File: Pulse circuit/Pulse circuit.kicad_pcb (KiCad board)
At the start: 4 copper layers, 8 parts, among them U1 module_max30102, U2 module_max30102, U3 DOIT-ESP32-DEVKIT-V1

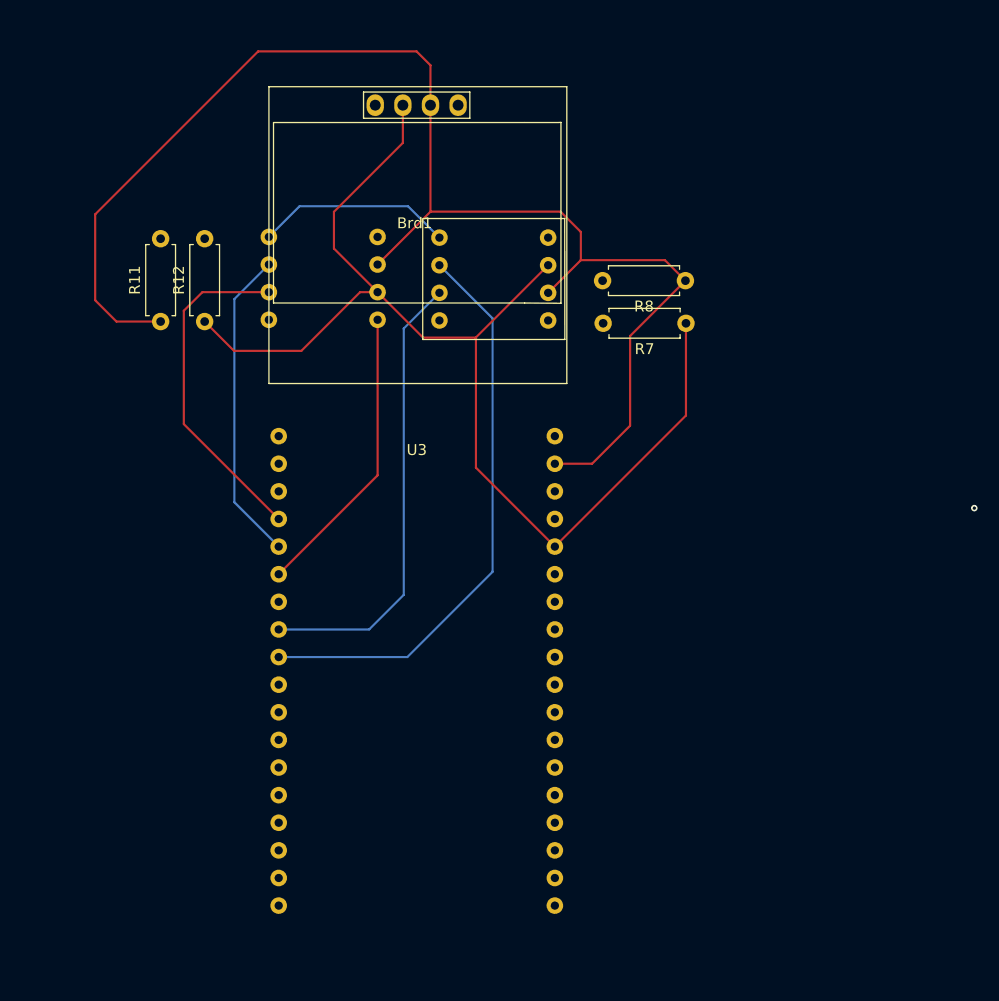
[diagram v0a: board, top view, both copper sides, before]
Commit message: Made some changes
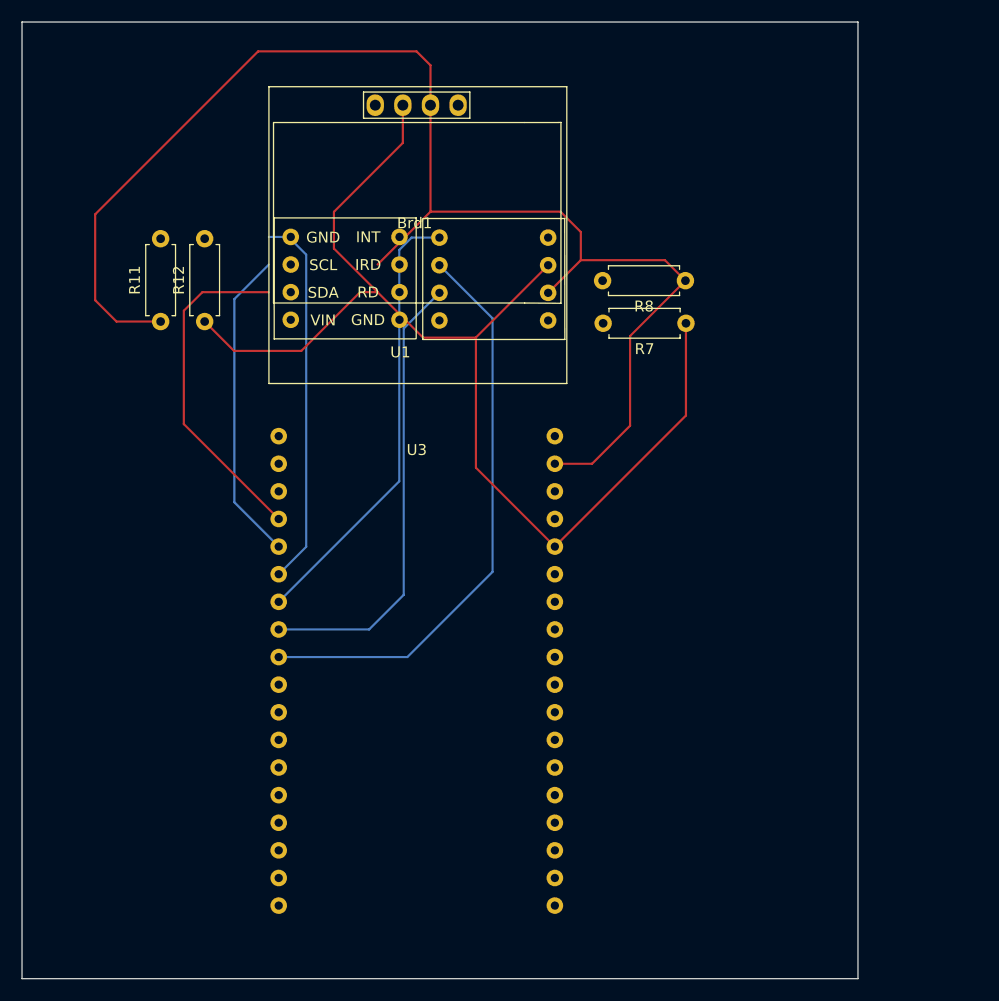
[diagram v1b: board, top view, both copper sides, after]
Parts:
- U1: moved to F.Cu
- moved U1 15.3 mm to (136.7, 74.7), turned to 0 degrees
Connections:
- U1 pad 8: INT5v -> INT3v3
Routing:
- net 5V: track 0.00 -> 73.2 mm, vias 3 -> 0
- net INT5v: track 18.1 -> 41.1 mm, vias 2 -> 0
- net INT3v3: track 27.2 -> 34.5 mm, vias 1 -> 0
- net RD5v: vias 2 -> 1
- net RD3v3: vias 2 -> 0
- net IRD5v: vias 2 -> 1
- net IRD3v3: vias 2 -> 0
- net GND: vias 5 -> 0
- net 3V3: vias 3 -> 0
- net (no net): vias 1 -> 0
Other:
- board outline added: 76.9 x 88 mm
